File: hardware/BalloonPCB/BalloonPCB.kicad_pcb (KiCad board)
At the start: 2 copper layers, 76.2 x 76.2 mm, 13 parts, among them P1 BMP180_HEADER, P2 GPS_HEADER, P3 ACCEL_HEADER, P4 CONN_01X24, P5 CONN_01X24, P6 5VDC_HEADER, P7 SMA, U1 Teensy3.5, U2 HX1

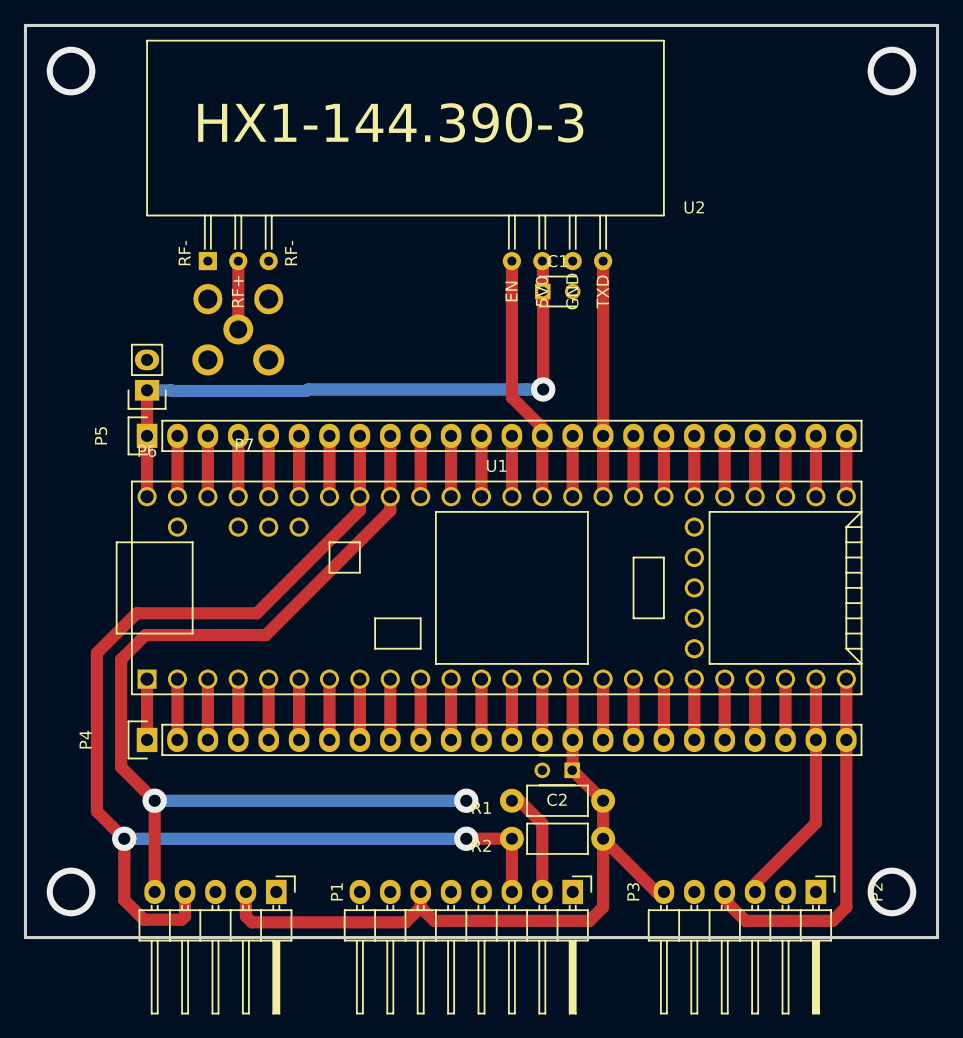
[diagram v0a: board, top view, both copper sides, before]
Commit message: Add pours
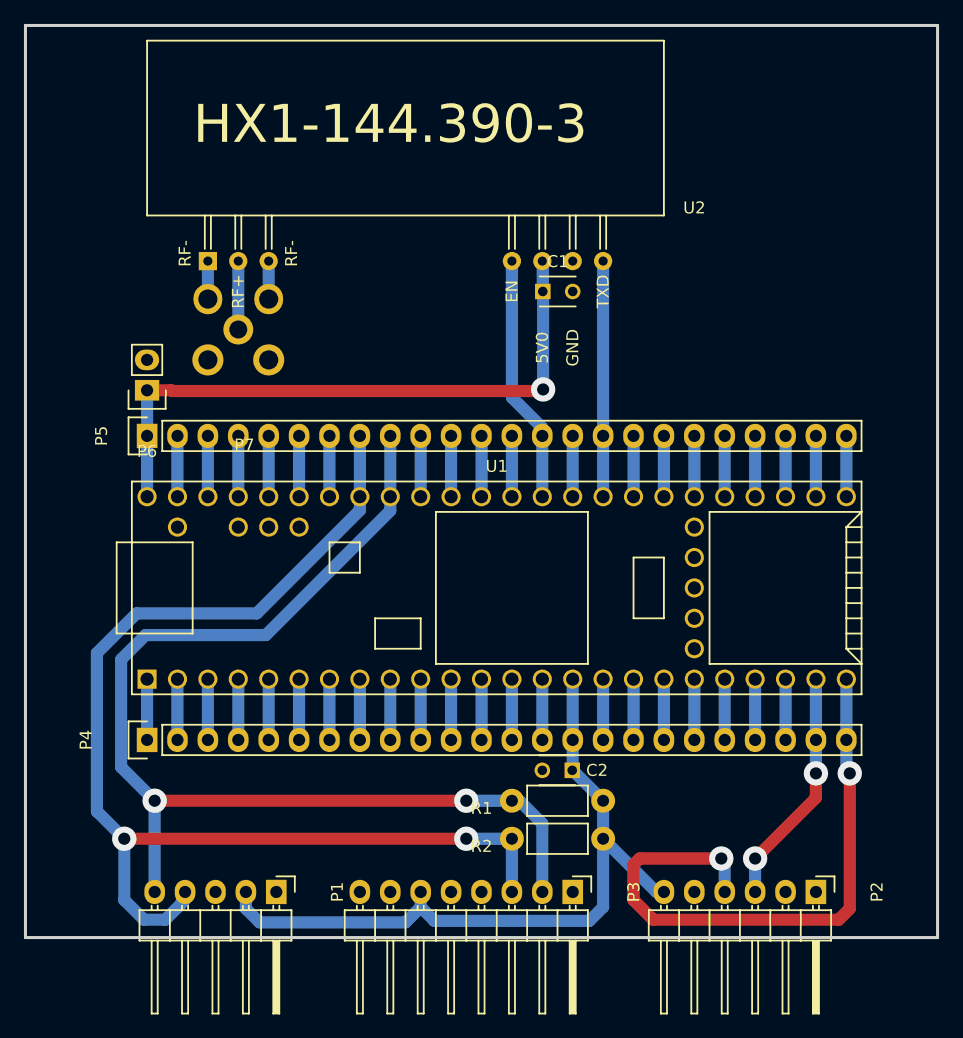
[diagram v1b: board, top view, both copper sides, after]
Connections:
- P7 pad 2: RF- -> GND
- U2 pad 1: RF- -> GND
- U2 pad 3: RF- -> GND
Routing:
- net GPS_RXD: track 31.1 -> 51.8 mm, vias 0 -> 2
- net GND: track 10.2 -> 16.5 mm
- net SDA0: track 89.7 -> 93.5 mm
- net SCL0: track 99.6 -> 98.8 mm
- net GPS_TXD: track 20.5 -> 21.2 mm, vias 0 -> 2
- net (no net): vias 4 -> 0
- added copper zone on B.Cu, net GND
